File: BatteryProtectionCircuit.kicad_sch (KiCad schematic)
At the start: 26 parts, among them J1 Conn_01x07_Pin, Q1 NMOS, U1 LMC555xN, U2 LM358, U3 LM358, U4 LM321

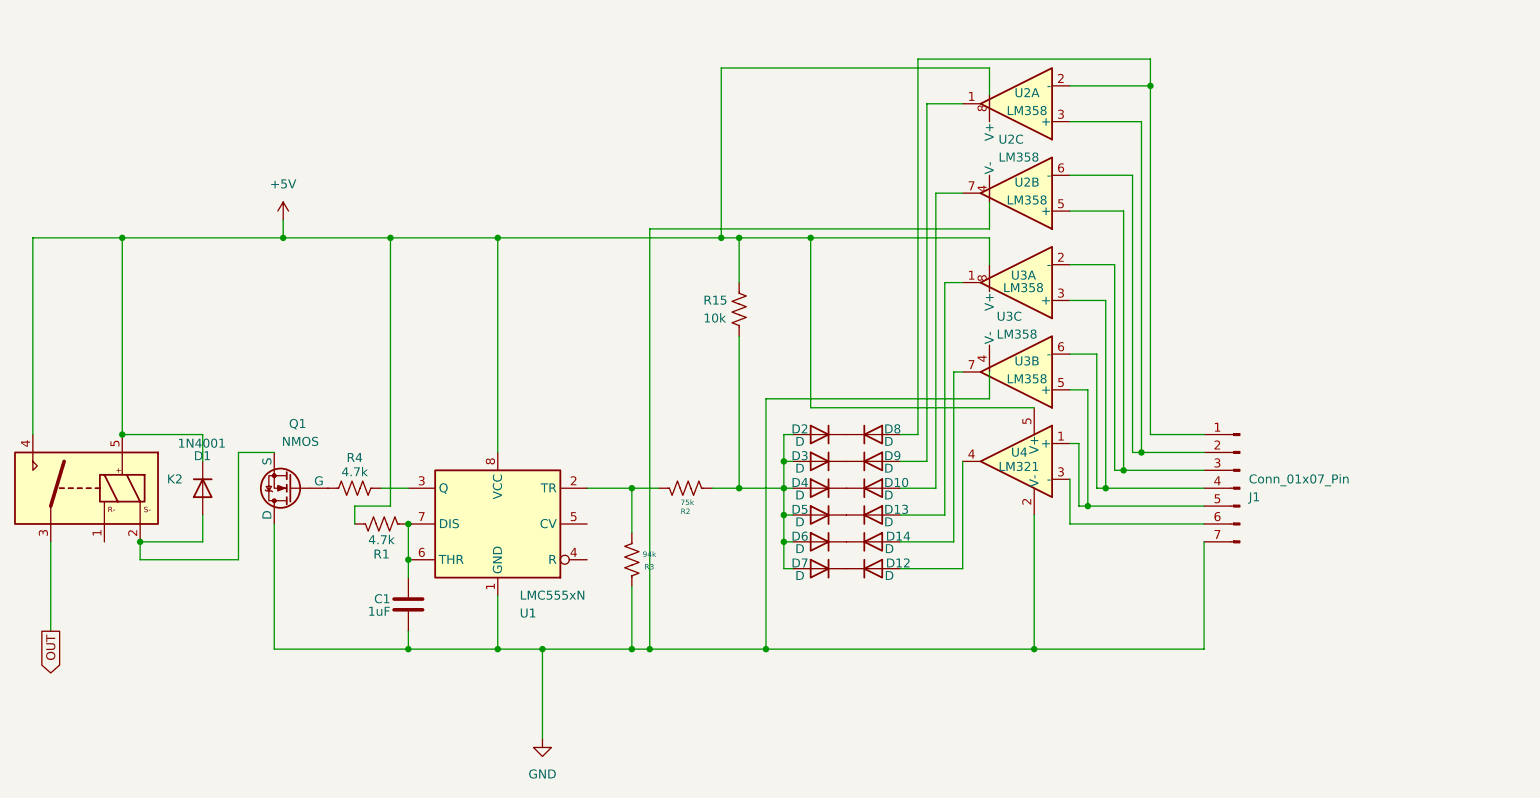
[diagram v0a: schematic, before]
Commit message: Update BatteryProtectionCircuit.kicad_sch
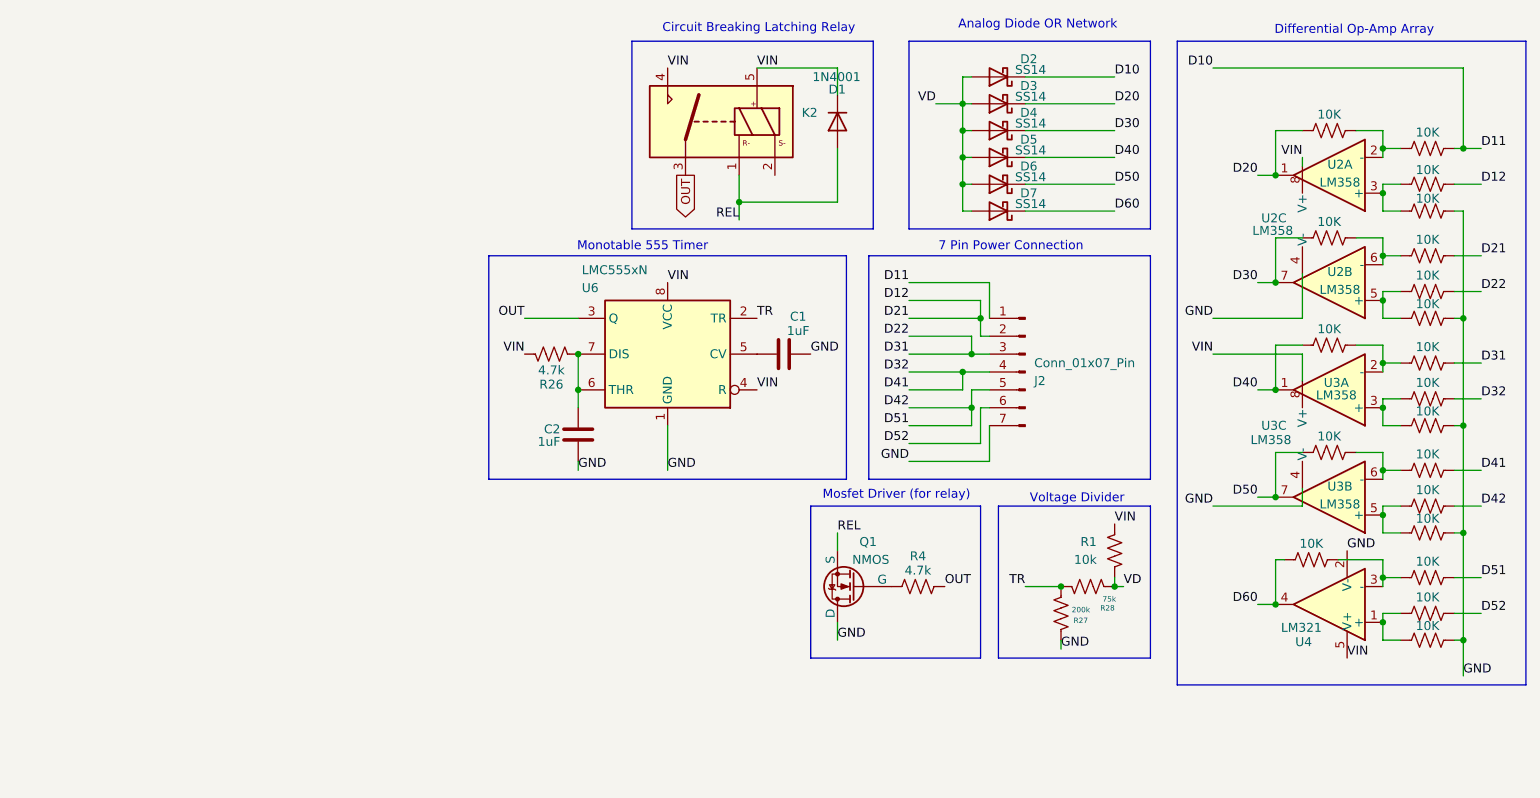
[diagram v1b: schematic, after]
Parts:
- removed D10, D12, D13, D2, D3, D4, D5, D6, D7, D8, D9: D, Diode_SMD:D_0805_2012Metric, symbol Device:D
- removed D14: D, Connector_PinHeader_1.00mm:PinHeader_1x02_P1.00mm_Vertical_SMD_Pin1Left, symbol Device:D
- removed J1: Conn_01x07_Pin, Connector_JST:JST_XH_B7B-XH-AM_1x07_P2.50mm_Vertical, symbol Connector:Conn_01x07_Pin
- removed R15: 10k, Resistor_SMD:R_0805_2012Metric, symbol Device:R_US
- removed R2: 75k, Resistor_SMD:R_0805_2012Metric, symbol Device:R_US
- removed R3: 94k, Resistor_SMD:R_0805_2012Metric, symbol Device:R_US
- removed U1: LMC555xN, Package_DIP:DIP-8_W7.62mm, symbol Timer:LMC555xN
- added C2: 1uF, Capacitor_SMD:C_0805_2012Metric, symbol Device:C
- added D2, D3, D4, D5, D6, D7: SS14, Diode_SMD:D_SMA, symbol Diode:SS14
- added J2: Conn_01x07_Pin, Connector_JST:JST_XH_B7B-XH-AM_1x07_P2.50mm_Vertical, symbol Connector:Conn_01x07_Pin
- added R10, R11, R12, R13, R14, R16, R17, R18, R19, R20, R21, R22, R23, R24, R25, R5, R6, R7, R8, R9: 10K, Resistor_SMD:R_0805_2012Metric, symbol Device:R_US
- added R26: 4.7k, Resistor_SMD:R_0805_2012Metric, symbol Device:R_US
- added R27: 200k, Resistor_SMD:R_0805_2012Metric, symbol Device:R_US
- added R28: 75k, Resistor_SMD:R_0805_2012Metric, symbol Device:R_US
- added U6: LMC555xN, Package_DIP:DIP-8_W7.62mm, symbol Timer:LMC555xN
- K2: footprint (none) -> Relay_THT:Relay_SPDT_Panasonic_DR-L
- R1: value 4.7k -> 10k
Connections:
- net GND: now also C1.2, C2.1, J2.7 (Pin_7), R12.2, R16.2, R19.2, R22.2, R27.1, R8.2, U6.1 (GND); no longer C1.1
- net OUT: now also R4.1, U6.3 (Q)
- net REL: now reaches D1.2 (A), Q1.3 (S)
- net REL: now also K2.1; no longer K2.2
- net at U3.5 (+): now also R18.1, R19.1; no longer U4.1 (+)
- net at U3.3 (+): now also R14.1, R16.1; no longer U3.6 (-)
- net D50: now reaches U3.7
- net D50: now also D6.1 (K), R24.1
- net at U4.3 (-): now also R20.1, R25.2
- net D60: now reaches U4.4
- net D60: now also D7.1 (K), R25.1
- net at U2.5 (+): now also R11.1, R12.1; no longer U3.2 (-)
- net at U2.3 (+): now also R7.1, R8.1; no longer U2.6 (-)
- net D30: now reaches U2.7
- net D30: now also D4.1 (K), R10.1
- net at U2.2 (-): now also R5.1, R6.2
- net VD: now reaches R1.2
- net VD: now also D2.2 (A), D3.2 (A), D4.2 (A), D5.2 (A), D6.2 (A), D7.2 (A), R28.2; no longer C1.2
- net D40: now reaches U3.1
- net D40: now also D5.1 (K), R23.1
- net D20: now reaches U2.1
- net D20: now also D3.1 (K), R6.1
- net +5V renamed VIN
- net VIN: now also R26.1, U6.4 (R), U6.8 (VCC)
- new net: R17.1, R24.2, U3.6 (-)
- new net: C1.1, U6.5 (CV)
- new net: R21.1, R22.1, U4.1 (+)
- new net: R10.2, R9.1, U2.6 (-)
- new net: R13.1, R23.2, U3.2 (-)
- new net: C2.2, R26.2, U6.6 (THR), U6.7 (DIS)
- new net D10: D2.1 (K), J2.1 (Pin_1), R5.2
- new net D12: J2.2 (Pin_2), R7.2, R9.2
- new net D22: J2.3 (Pin_3), R11.2, R13.2
- new net D32: J2.4 (Pin_4), R14.2, R17.2
- new net D42: J2.5 (Pin_5), R18.2, R20.2
- new net D52: J2.6 (Pin_6), R21.2
- new net TR: R27.2, R28.1, U6.2 (TR)
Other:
- note added: "7 Pin Power Connection"
- note added: "Analog Diode OR Network"
- note added: "Circuit Breaking Latching Relay"
- note added: "Differential Op-Amp Array"
- note added: "Monotable 555 Timer"
- note added: "Mosfet Driver (for relay)"
- note added: "Voltage Divider"
- moved on the sheet: D1, K2, Q1, R4, U2A, U2B, U2C, U3A, U3B, U3C, U4
